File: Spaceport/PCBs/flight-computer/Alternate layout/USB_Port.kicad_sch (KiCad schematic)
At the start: 5 parts, among them J4 USB_C_Receptacle_USB2.0_16P

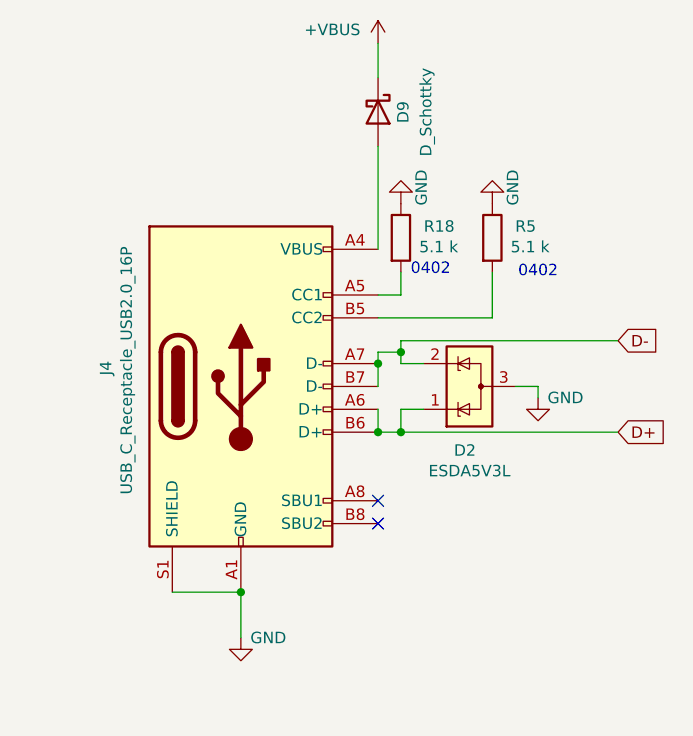
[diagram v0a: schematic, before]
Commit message: Restore flight computer files
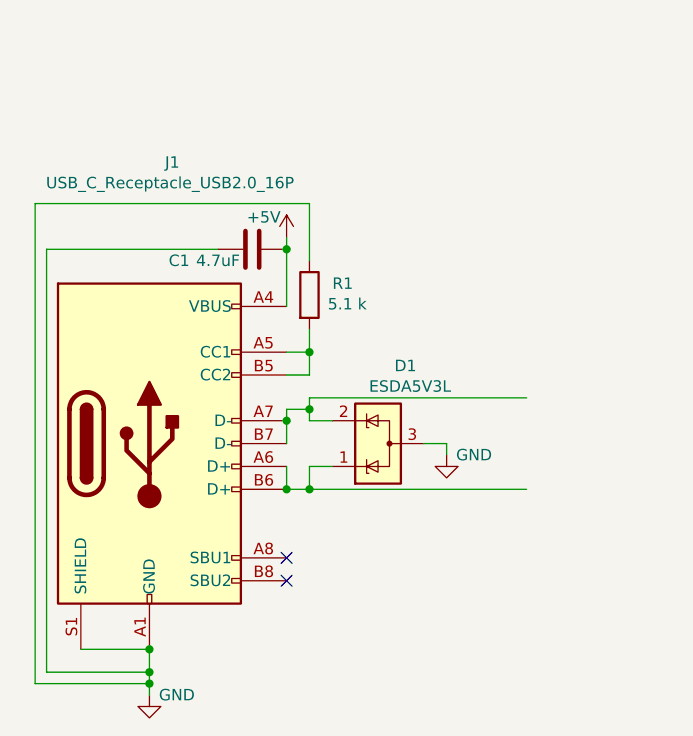
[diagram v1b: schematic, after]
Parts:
- removed D2: ESDA5V3L, Package_TO_SOT_SMD:SOT-23-3, symbol Power_Protection:ESDA5V3L
- removed D9: D_Schottky, Diode_SMD:D_0805_2012Metric_Pad1.15x1.40mm_HandSolder, symbol Device:D_Schottky
- removed J4: USB_C_Receptacle_USB2.0_16P, Connector_USB:USB_C_Receptacle_G-Switch_GT-USB-7010ASV, symbol Connector:USB_C_Receptacle_USB2.0_16P
- removed R18, R5: 5.1 k, Resistor_SMD:R_0603_1608Metric_Pad0.98x0.95mm_HandSolder, symbol Device:R
- added C1: 4.7uF, symbol Device:C
- added D1: ESDA5V3L, Package_TO_SOT_SMD:SOT-23-3, symbol Power_Protection:ESDA5V3L
- added J1: USB_C_Receptacle_USB2.0_16P, Connector_USB:USB_C_Receptacle_G-Switch_GT-USB-7010ASV, symbol Connector:USB_C_Receptacle_USB2.0_16P
- added R1: 5.1 k, symbol Device:R
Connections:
- net GND: now also C1.1, D1.3 (A), J1.A1 (GND), J1.A12 (GND), J1.B1 (GND), J1.B12 (GND), J1.S1 (SHIELD), R1.1
- new net: J1.A5 (CC1), J1.B5 (CC2), R1.2
- new net: D1.1 (K), J1.A6 (D+), J1.B6 (D+)
- new net: D1.2 (K), J1.A7 (D-), J1.B7 (D-)
- new net +5V: C1.2, J1.A4 (VBUS), J1.A9 (VBUS), J1.B4 (VBUS), J1.B9 (VBUS)
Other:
- note removed: "0402"
